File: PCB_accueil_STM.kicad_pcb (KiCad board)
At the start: 2 copper layers, 131 x 86 mm, 20 parts, among them J1 RJ12 Haut, J2 RJ12 Bas, J3 SparkFun Battery Babysitter, J4 RJ12 capteur, U1 module_mpu6050

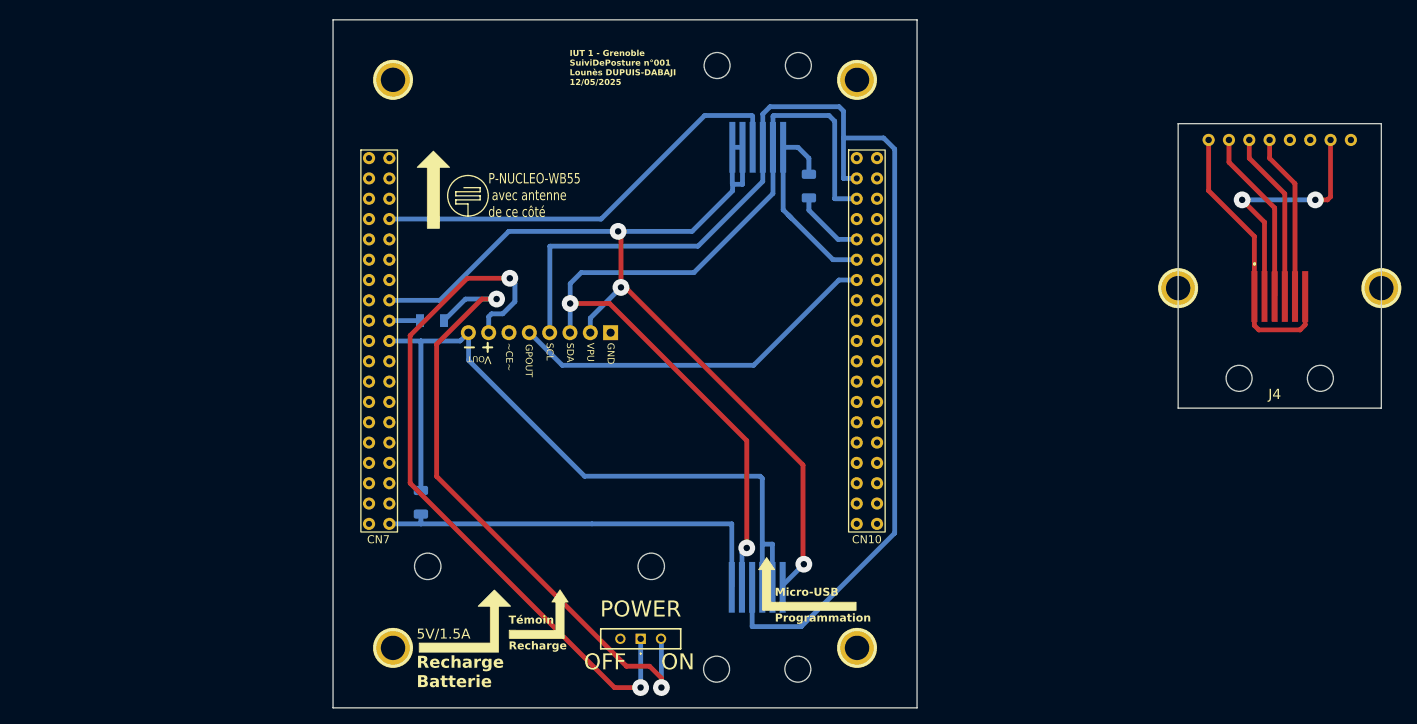
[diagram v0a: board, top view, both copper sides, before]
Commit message: rentrée scolaire
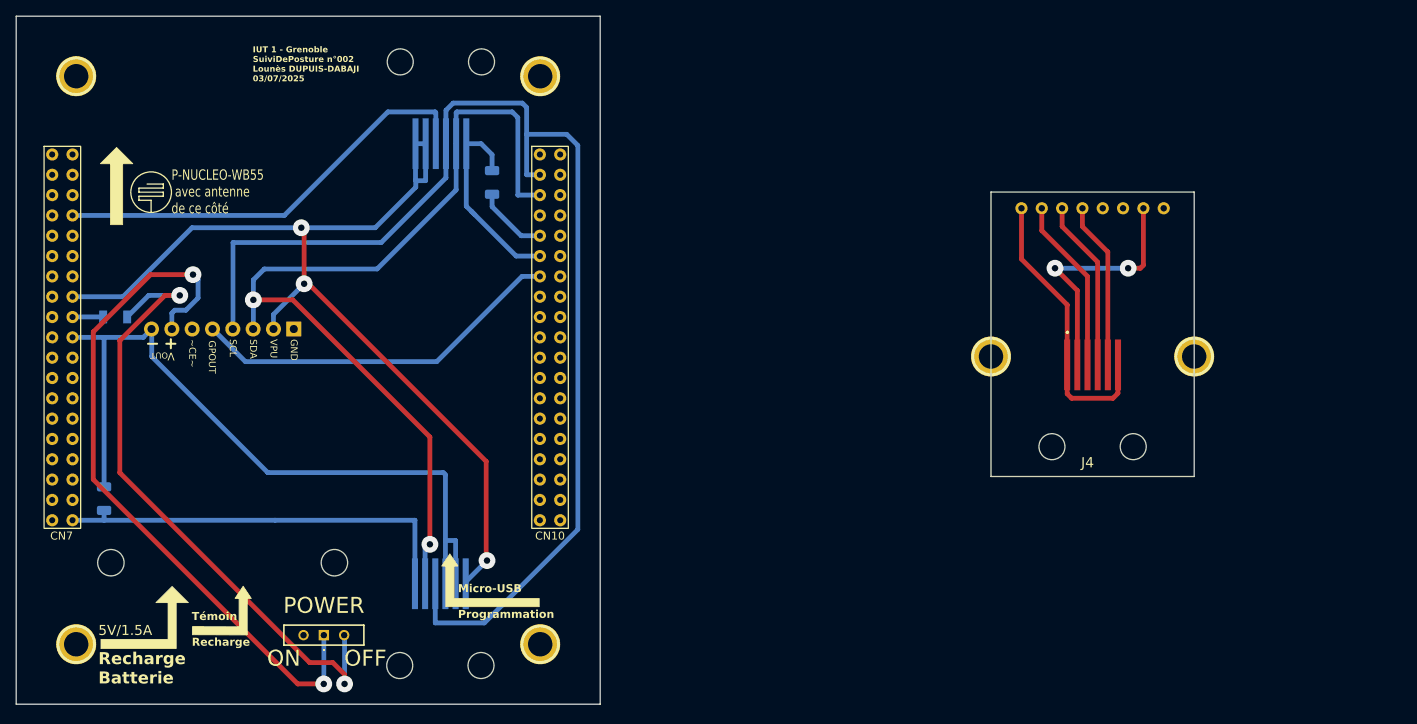
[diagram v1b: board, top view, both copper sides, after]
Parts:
- moved 1PIN 39.6 mm to (86.4, 131.7)
- moved 1PIN 39.6 mm to (86.4, 60.7)
- moved ? 39.6 mm to (122.4, 74.5) (x2)
- moved D1 39.6 mm to (91.3, 90.8)
- moved J3 39.6 mm to (104.1, 107.4)
- moved R2 39.6 mm to (89.9, 113.5)
- moved S1 39.6 mm to (117.4, 130.6)
- moved 1PIN 39.6 mm to (144.4, 131.7)
- moved 1PIN 39.6 mm to (144.4, 60.7)
- moved CN10 39.6 mm to (108.8, 98.5)
- moved CN7 39.6 mm to (108.8, 98.5)
- moved J1 39.6 mm to (132.0, 59.0)
- moved J2 39.6 mm to (131.9, 134.4)
- moved R1 39.6 mm to (138.4, 74.0)
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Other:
- board size 131 x 86 mm -> 147.2 x 86 mm
- board text added: "IUT 1 - Grenoble SuiviDePosture n°002 Lounès DUPUIS-DABAJI 03/07/2025"
- board text added: "SuiviDePosture n°003 DUPUIS-DABAJI Lounès (Projet FAME) 03/07/2025"
- board text removed: "IUT 1 - Grenoble SuiviDePosture n°001 Lounès DUPUIS-DABAJI 12/05/2025"
- board text removed: "SuiviDePosture n°002 DUPUIS-DABAJI Lounès (Projet FAME) 12/05/2025"
